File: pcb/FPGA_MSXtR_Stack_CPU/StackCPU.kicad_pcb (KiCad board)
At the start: 2 copper layers, 95.2 x 65.4 mm, 61 parts, among them J1 I2S_CONN, J2 SOUNDIN, J3 Conn_02x06_Odd_Even, J4 GND, Q1 NMOS, Q2 NMOS, Q3 NMOS

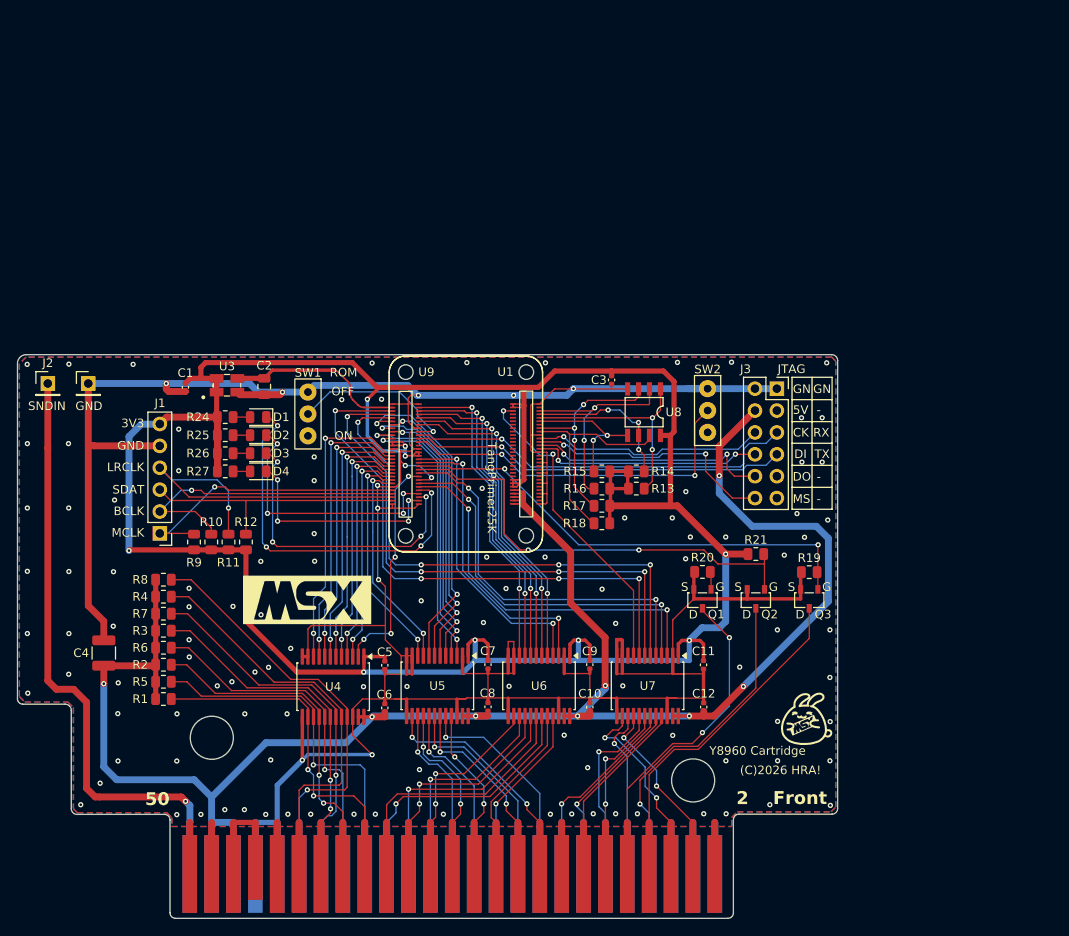
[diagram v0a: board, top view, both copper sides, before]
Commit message: Updated
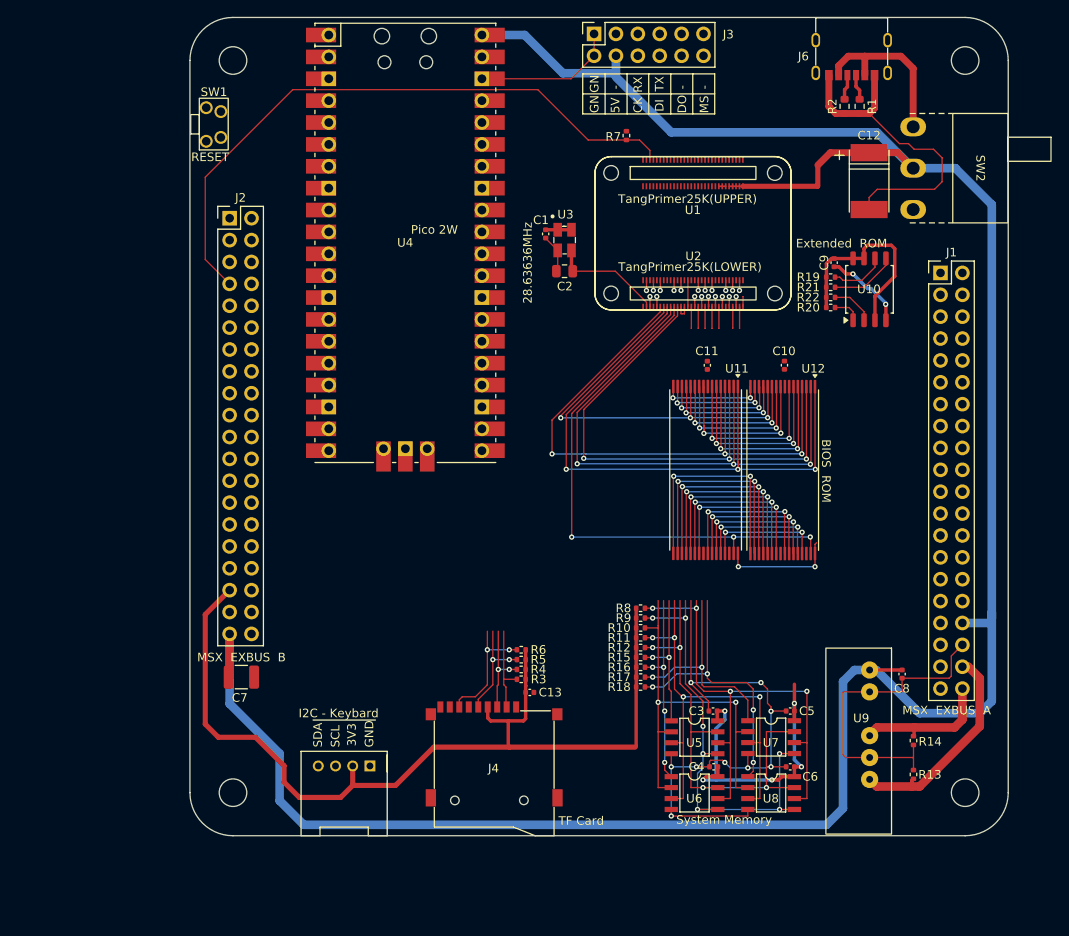
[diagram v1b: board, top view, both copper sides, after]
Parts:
- removed D1, D2, D3, D4: LED, LED_SMD:LED_0805_2012Metric
- removed G1: LOGO, 0-My_Parts:msx_logo_15x5p8
- removed G2: LOGO, 0-My_Parts:usa_10x7
- removed Q1, Q2, Q3: NMOS, 0-My_Parts:MOSFET(SMD)
- removed R24, R25, R26, R27: 470, Resistor_SMD:R_0805_2012Metric
- added C13: 0.1uF, Capacitor_SMD:C_0402_1005Metric, F.Cu at (122.3, 107.0)
- added J5: Keybard I2C Connector, 0-My_Parts:Grove_I2C, F.Cu at (103.7, 115.5)
- added J6: USB_C_Receptacle_PowerOnly_6P, 0-My_Parts:USB-C(C2927029), F.Cu at (159.6, 31.3)
- added R22: 3.3K, Resistor_SMD:R_0402_1005Metric, F.Cu at (157.2, 61.1)
- added REF**: MSXtR Stack Base, My Parts:MSXtR Stack Base, F.Cu at (82.8, 123.6)
- added U10: W25Q32JVSS, Package_SO:SOIC-8_5.3x5.3mm_P1.27mm, F.Cu at (161.7, 60.2)
- added U11: ~, Package_SO:TSOP-I-32_18.4x8mm_P0.5mm, F.Cu at (142.7, 81.1)
- added U12: ~, Package_SO:TSOP-I-32_18.4x8mm_P0.5mm, F.Cu at (151.6, 81.2)
- C12: value 0.1uF -> 470uF; footprint Capacitor_SMD:C_0402_1005Metric -> My Parts:Capacitor(C453487)
- C4: value 100uF -> 0.1uF; footprint Capacitor_SMD:C_1210_3225Metric -> Capacitor_SMD:C_0402_1005Metric
- C7: value 0.1uF -> 100uF; footprint Capacitor_SMD:C_0402_1005Metric -> Capacitor_SMD:C_1210_3225Metric
- C8: value 0.1uF -> 1uF
- J1: value I2S_CONN -> MSX_EXBUS_A; footprint Connector_PinHeader_2.54mm:PinHeader_1x06_P2.54mm_Vertical -> Connector_PinHeader_2.54mm:PinHeader_2x20_P2.54mm_Vertical
- J2: value SOUNDIN -> MSX_EXBUS_B; footprint Connector_PinHeader_2.54mm:PinHeader_1x01_P2.54mm_Vertical -> Connector_PinHeader_2.54mm:PinHeader_2x20_P2.54mm_Vertical
- J4: value GND -> Micro_SD_Card; footprint Connector_PinHeader_2.54mm:PinHeader_1x01_P2.54mm_Vertical -> 0-My_Parts:MicroSD(C91145)
- R1, R2: value 4.7k -> 5.1K; footprint Resistor_SMD:R_0805_2012Metric -> Resistor_SMD:R_0603_1608Metric
- R10, R11, R12, R19, R21, R9: value 3.3k -> 3.3K; footprint Resistor_SMD:R_0805_2012Metric -> Resistor_SMD:R_0402_1005Metric
- R13, R14: value 4.7k -> 100K; footprint Resistor_SMD:R_0805_2012Metric -> Resistor_SMD:R_0402_1005Metric
- R15, R16, R17, R18, R7, R8: value 4.7k -> 3.3K; footprint Resistor_SMD:R_0805_2012Metric -> Resistor_SMD:R_0402_1005Metric
- R20: value 10k -> 3.3K; footprint Resistor_SMD:R_0805_2012Metric -> Resistor_SMD:R_0402_1005Metric
- R3, R4, R5, R6: value 4.7k -> 22K; footprint Resistor_SMD:R_0805_2012Metric -> Resistor_SMD:R_0402_1005Metric
- SW1: value ~ -> SW_MEC_5G; footprint 0-My_Parts:SlideSwitch -> My Parts:SideSW (C2906286)
- SW2: value ~ -> SW_SPDT; footprint 0-My_Parts:SlideSwitch -> My Parts:Slide SW(C7431058)
- U1: footprint 0-My_Parts:TangPrimer25K(UPPER) -> My Parts:TangPrimer25K(UPPER)
- U2: footprint 0-My_Parts:MSX Cartridge_1 -> My Parts:TangPrimer25K(LOWER)
- U3: footprint 0-My_Parts:CLOCK -> My Parts:CLOCK
- U4: footprint Package_SO:SSOP-24_5.3x8.2mm_P0.65mm -> MCU_RaspberryPi_and_Boards:RPi_Pico_SMD_TH
- U5, U6, U7: footprint Package_SO:SSOP-24_5.3x8.2mm_P0.65mm -> My Parts:QSPI-SRAM 4Mbit (8SOIC)
- U8: footprint 0-My_Parts:QSPI-SRAM 4Mbit (8SOIC) -> My Parts:QSPI-SRAM 4Mbit (8SOIC)
- U9: footprint 0-My_Parts:TangPrimer25K(LOWER) -> My Parts:DCDC_MAU108
- moved R1 106.1 mm to (160.6, 38.9), turned to -90 degrees
- moved R2 102.3 mm to (158.8, 38.9), turned to -90 degrees
- moved J1 95.6 mm to (169.9, 58.3), turned to 0 degrees
- moved U2 91.1 mm to (141.2, 53.6)
- moved R7 77.3 mm to (133.5, 42.3), turned to -90 degrees
- moved C4 72.0 mm to (143.6, 115.6), turned to 180 degrees
- moved C12 64.0 mm to (161.7, 47.6), turned to 0 degrees
- moved J4 63.4 mm to (118.1, 113.5)
- moved U9 57.1 mm to (161.7, 112.0)
- moved R8 55.5 mm to (135.1, 97.2)
- moved C9 54.6 mm to (157.6, 57.1)
- moved R9 52.6 mm to (135.1, 98.3), turned to 0 degrees
- moved U4 52.2 mm to (107.8, 54.8), turned to 0 degrees
- moved R10 50.8 mm to (135.1, 99.5), turned to 0 degrees
- moved R11 49.1 mm to (135.1, 100.6), turned to 180 degrees
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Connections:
- C10 pad 1: GND -> +3V3
- C10 pad 2: +5V -> GND
- C11 pad 1: GND -> +3V3
- C11 pad 2: +3V3 -> GND
- C12 pad 1: GND -> +5V
- C12 pad 2: +5V -> GND
- C4 pad 1: +5V -> +3V3
- C5 pad 1: GND -> +3V3
- C5 pad 2: +3V3 -> GND
- C6 pad 1: GND -> +3V3
- C6 pad 2: +5V -> GND
- C7 pad 1: GND -> +5V
- C7 pad 2: +3V3 -> GND
- C8 pad 1: GND -> +5V
- C8 pad 2: +5V -> GND
- J1 pad 1: AUDIO_MCLK -> SLOT_CS2_N
- J1 pad 2: AUDIO_BCLK -> SLOT_RFSH_N
- J1 pad 3: AUDIO_SDATA -> SLOT_SLTSL1_N
- J1 pad 4: AUDIO_LRCLK -> SLOT_SLTSL0_N
- J1 pad 5: GND -> SLOT_SLTSL2_N
- J1 pad 6: +3V3 -> SLOT_SLTSL3_N
- J2 pad 1: Net-(J2-Pin_1) -> unconnected-(J2-Pin_1-Pad1)
- J4 pad 1: GND -> unconnected-(J4-DAT2-Pad1)
- R1 pad 1: +5V -> Net-(J6-CC1)
- R1 pad 2: D0 -> GND
- R10 pad 2: AUDIO_BCLK -> SRAM_SIO1
- R11 pad 1: +3V3 -> SRAM_SIO2
- R11 pad 2: AUDIO_LRCLK -> +3V3
- R12 pad 1: +3V3 -> SRAM_SIO3
- R12 pad 2: AUDIO_SDATA -> +3V3
- R13 pad 1: +3V3 -> GND
- R13 pad 2: SRAM_CS_N -> +12V
- R14 pad 1: +3V3 -> -12V
- R14 pad 2: SRAM_SCLK -> GND
- R15 pad 1: +3V3 -> SRAM_CS0_N
- R15 pad 2: SRAM_SIO0 -> +3V3
- R16 pad 1: +3V3 -> SRAM_CS1_N
- R16 pad 2: SRAM_SIO1 -> +3V3
- R17 pad 1: SRAM_SIO2 -> SRAM_CS2_N
- R18 pad 1: SRAM_SIO3 -> SRAM_CS3_N
- R19 pad 1: SLOT_INTR -> SROM_SCLK
- R19 pad 2: GND -> +3V3
- R2 pad 1: +5V -> Net-(J6-CC2)
- R2 pad 2: D2 -> GND
- R20 pad 1: SLOT_DATA_DIR -> SROM_CS_N
- R20 pad 2: GND -> +3V3
- R21 pad 1: +3V3 -> SROM_MOSI
- R21 pad 2: SLOT_WAIT -> +3V3
- R3 pad 1: +5V -> SD_SPI_CS_N
- R3 pad 2: D4 -> +3V3
- R4 pad 1: +5V -> SD_SPI_MOSI
- R4 pad 2: D6 -> +3V3
- R5 pad 1: +5V -> SD_SPI_SCK
- R5 pad 2: D1 -> +3V3
- R6 pad 1: +5V -> SD_SPI_MISO
- R6 pad 2: D3 -> +3V3
- R7 pad 1: +5V -> +3V3
- R7 pad 2: D5 -> SLOT_OE_N
- R8 pad 1: +5V -> +3V3
- R8 pad 2: D7 -> SRAM_SCLK
- R9 pad 2: AUDIO_MCLK -> SRAM_SIO0
- SW1 pad 1: GND -> RESET_BUTTON
- SW1 pad 2: DIPSW0 -> RESET_BUTTON
- SW2 pad 1: GND -> Net-(SW2-A)
- SW2 pad 2: DIPSW1 -> +5V
- U1 pad 10: unconnected-(U1-N/A-Pad10) -> SLOT_CS1_N
- U1 pad 11: SRAM_SIO0 -> SRAM_SIO1
- U1 pad 12: unconnected-(U1-N/A-Pad12) -> SLOT_CS2_N
- U1 pad 14: unconnected-(U1-N/A-Pad14) -> MCU_CS_N
- U1 pad 16: unconnected-(U1-N/A-Pad16) -> MCU_SCLK
- U1 pad 18: unconnected-(U1-hs_cs_n-Pad18) -> MCU_MOSI
- U1 pad 20: unconnected-(U1-hs_miso3-Pad20) -> MCU_MISO
- U1 pad 22: unconnected-(U1-hs_clk-Pad22) -> SRAM_CS0_N
- U1 pad 24: unconnected-(U1-hs_miso2-Pad24) -> SRAM_CS1_N
- U1 pad 26: unconnected-(U1-hs_miso1-Pad26) -> SRAM_CS2_N
- U1 pad 28: unconnected-(U1-hs_miso0-Pad28) -> SRAM_CS3_N
- U1 pad 3: unconnected-(U1-N/A-Pad3) -> SLOT_M1_N
- U1 pad 30: unconnected-(U1-hs_mosi3-Pad30) -> SLOT_SLTSL0_N
- U1 pad 32: unconnected-(U1-hs_mosi2-Pad32) -> SLOT_SLTSL1_N
- U1 pad 34: unconnected-(U1-hs_mosi1-Pad34) -> SLOT_SLTSL2_N
- U1 pad 36: unconnected-(U1-hs_mosi0-Pad36) -> SLOT_SLTSL3_N
- U1 pad 5: SRAM_SIO1 -> SLOT_OE_N
- U1 pad 6: SLOT_M1_N -> SLOT_DATA_DIR
- U1 pad 8: unconnected-(U1-N/A-Pad8) -> SLOT_ROM0_CE_N
- U1 pad 9: SRAM_CS_N -> SRAM_SIO0
- U4 pad 1: +3V3 -> unconnected-(U4-GP0-Pad1)
- U4 pad 10: SLOT_D0 -> MCU_MOSI
- U4 pad 11: GND -> SD_SPI_MISO
- U4 pad 12: GND -> SD_SPI_CS_N
- U4 pad 14: D0 -> SD_SPI_SCK
- U4 pad 15: D1 -> SD_SPI_MOSI
- U4 pad 16: D2 -> unconnected-(U4-GP12-Pad16)
- U4 pad 17: D3 -> unconnected-(U4-GP13-Pad17)
- U4 pad 18: D4 -> GND
- U4 pad 19: D5 -> unconnected-(U4-GP14-Pad19)_1
- U4 pad 2: SLOT_BUSDIR -> unconnected-(U4-GP1-Pad2)
- U4 pad 20: D6 -> unconnected-(U4-GP15-Pad20)
- U4 pad 21: D7 -> DIPSW3
- U4 pad 22: GND -> DIPSW2
- U4 pad 23: +5V -> GND
- U4 pad 24: +5V -> DIPSW1
- U4 pad 3: SLOT_D7 -> unconnected-(U4-GND-Pad3)_1
- U4 pad 4: SLOT_D6 -> unconnected-(U4-GP2-Pad4)_1
- U4 pad 5: SLOT_D5 -> MCU_INTR
- U4 pad 6: SLOT_D4 -> MCU_MISO
- U4 pad 7: SLOT_D3 -> MCU_CS_N
- U4 pad 8: SLOT_D2 -> GND
- U4 pad 9: SLOT_D1 -> MCU_SCLK
- U5 pad 1: +3V3 -> SRAM_CS0_N
- U5 pad 2: GND -> SRAM_SIO1
- U5 pad 3: SLOT_A8 -> SRAM_SIO2
- U5 pad 4: SLOT_A9 -> GND
- U5 pad 5: SLOT_A10 -> SRAM_SIO0
- U5 pad 6: SLOT_A11 -> SRAM_SCLK
- U5 pad 7: SLOT_A12 -> SRAM_SIO3
- U5 pad 8: SLOT_A13 -> +3V3
- U6 pad 1: +3V3 -> SRAM_CS1_N
- U6 pad 2: GND -> SRAM_SIO1
- U6 pad 3: SLOT_A7 -> SRAM_SIO2
- U6 pad 4: SLOT_A6 -> GND
- U6 pad 5: SLOT_A5 -> SRAM_SIO0
- U6 pad 6: SLOT_A4 -> SRAM_SCLK
- U6 pad 7: SLOT_A3 -> SRAM_SIO3
- U6 pad 8: SLOT_A2 -> +3V3
- U7 pad 1: +3V3 -> SRAM_CS2_N
- U7 pad 2: GND -> SRAM_SIO1
- U7 pad 3: SLOT_RD_N -> SRAM_SIO2
- U7 pad 4: SLOT_WR_N -> GND
- U7 pad 5: SLOT_RESET_N -> SRAM_SIO0
- U7 pad 6: SLOT_MERQ_N -> SRAM_SCLK
- U7 pad 7: SLOT_IORQ_N -> SRAM_SIO3
- U7 pad 8: SLOT_SLTSL_N -> +3V3
- U8 pad 1: SRAM_CS_N -> SRAM_CS3_N
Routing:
- net GND: track 415.5 -> 177.0 mm, vias 117 -> 11
- net +3V3: track 302.4 -> 177.2 mm, vias 9 -> 5
- net +5V: track 215.3 -> 291.1 mm, vias 8 -> 0
- net SLOT_OE_N: track 0.00 -> 73.4 mm
- net SLOT_SLTSL_N: track 66.3 -> 0.00 mm, vias 4 -> 0
- net Net-(J2-Pin_1): track 64.8 -> 0.00 mm, vias 1 -> 0
- net SLOT_IORQ_N: track 64.3 -> 0.00 mm, vias 4 -> 0
- net SLOT_MERQ_N: track 62.7 -> 1.19 mm, vias 4 -> 1
- net SLOT_INTR: track 55.5 -> 0.00 mm, vias 2 -> 0
- net SLOT_WAIT: track 52.4 -> 0.00 mm, vias 2 -> 0
- net D7: track 44.7 -> 0.00 mm, vias 1 -> 0
- net UART_RX: track 45.7 -> 1.19 mm
- net SLOT_RESET_N: track 45.3 -> 1.18 mm, vias 2 -> 1
- net UART_TX: track 43.8 -> 0.00 mm, vias 1 -> 0
- net Net-(D1-K): track 43.3 -> 0.00 mm, vias 4 -> 0
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- removed copper zone on B.Cu, net GND
- removed copper zone on F.Cu, net GND
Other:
- board size 95.2 x 65.4 mm -> 95 x 95 mm
- board text added: "28.63636MHz"
- board text added: "BIOS ROM"
- board text added: "Extended ROM"
- board text added: "I2C - Keybard"
- board text added: "Pico 2W"
- board text added: "RESET"
- board text added: "System Memory"
- board text added: "TF Card"
- board text removed: "(C)2026 HRA!"
- board text removed: "3V3"
- board text removed: "BCLK"
- board text removed: "GND"
- board text removed: "JTAG"
- board text removed: "LRCLK"
- board text removed: "MCLK"
- board text removed: "OFF"
- board text removed: "ON"
- board text removed: "Prototype Rev.1"
- board text removed: "ROM"
- board text removed: "SDAT"
- board text removed: "SNDIN"
- board text removed: "TangPrimer25K"
- board text removed: "Y8960 Cartridge"
